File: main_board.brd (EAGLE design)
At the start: 201.2 x 155.4 mm, 206 parts, among them IC10 MEGA48/88/168-PU, IC11 MEGA48/88/168-PU, IC2 LM567N, IC3 74AC11000D, IC4 4050D, IC5 ATMEGA644-20PU, IC6 4051D, IC7 AD8655R, IC8 4051D, IC9 TINY24/44/84-SSU, J1 22-27-2041-04, K2 4052, Q2 MOSFET-NCHANNELSMD, U1 XC9572VQ44

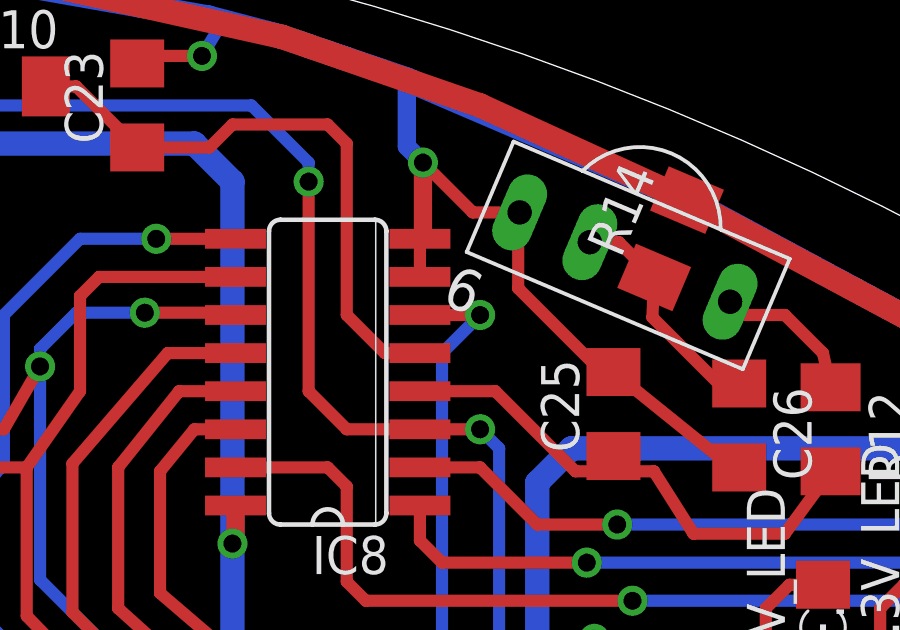
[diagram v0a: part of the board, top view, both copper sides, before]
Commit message: Main: Changed MUX-EN to MUX-INH. This pin should have been called INHIBIT  in the first place because it is LOW ACTIVE!!!!!
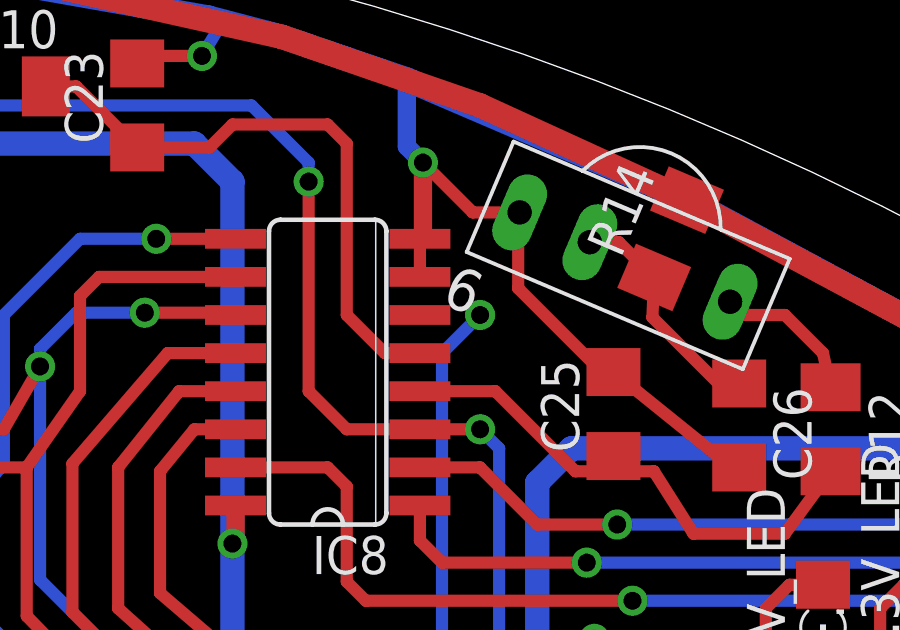
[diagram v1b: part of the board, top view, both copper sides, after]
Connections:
- net MUX1-EN renamed MUX1-INH
- new net MUX2-INH: IC8.6
- net MUX2-EN: no longer IC8.6
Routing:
- net MUX2-EN: track 73.1 -> 71.1 mm
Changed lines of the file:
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@@
 <via x="14.732" y="80.1878" extent="1-16" drill="0.6"/>
 </signal>
-<signal name="MUX1-EN">
+<signal name="MUX1-INH">
 <contactref element="IC6" pad="6"/>
 <contactref element="IC11" pad="12"/>
@@
 </signal>
 <signal name="MUX2-EN">
-<contactref element="IC8" pad="6"/>
 <contactref element="IC11" pad="13"/>
 <wire x1="41.91" y1="28.1178" x2="39.37" y2="28.1178" width="0.4064" layer="16"/>
@@
 <wire x1="38.1" y1="26.8478" x2="32.385" y2="26.8478" width="0.4064" layer="16"/>
 <wire x1="30.48" y1="28.7528" x2="30.48" y2="66.2178" width="0.4064" layer="1"/>
-<wire x1="29.7434" y1="86.5378" x2="31.75" y2="86.5378" width="0.4064" layer="1"/>
 <via x="31.75" y="86.5378" extent="1-16" drill="0.6"/>
 <wire x1="31.75" y1="86.5378" x2="30.48" y2="85.2678" width="0.4064" layer="16"/>
@@
 <wire x1="-7.62" y1="-6.985" x2="-9.525" y2="-6.985" width="0.4064" layer="16"/>
 </signal>
+<signal name="MUX2-INH">
+<contactref element="IC8" pad="6"/>
+</signal>
 </signals>
